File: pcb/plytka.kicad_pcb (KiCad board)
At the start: 2 copper layers, 27 x 78 mm, 51 parts, among them J1 Display, J2 Program, Q3 AO3400A, Q4 AO3400A, SW1 RESET, SW2 USER0, SW3 USER2, SW4 USER3, U1 TPS61022, U2 TP4054, U3 USBLC6-2P6, U4 CH340K

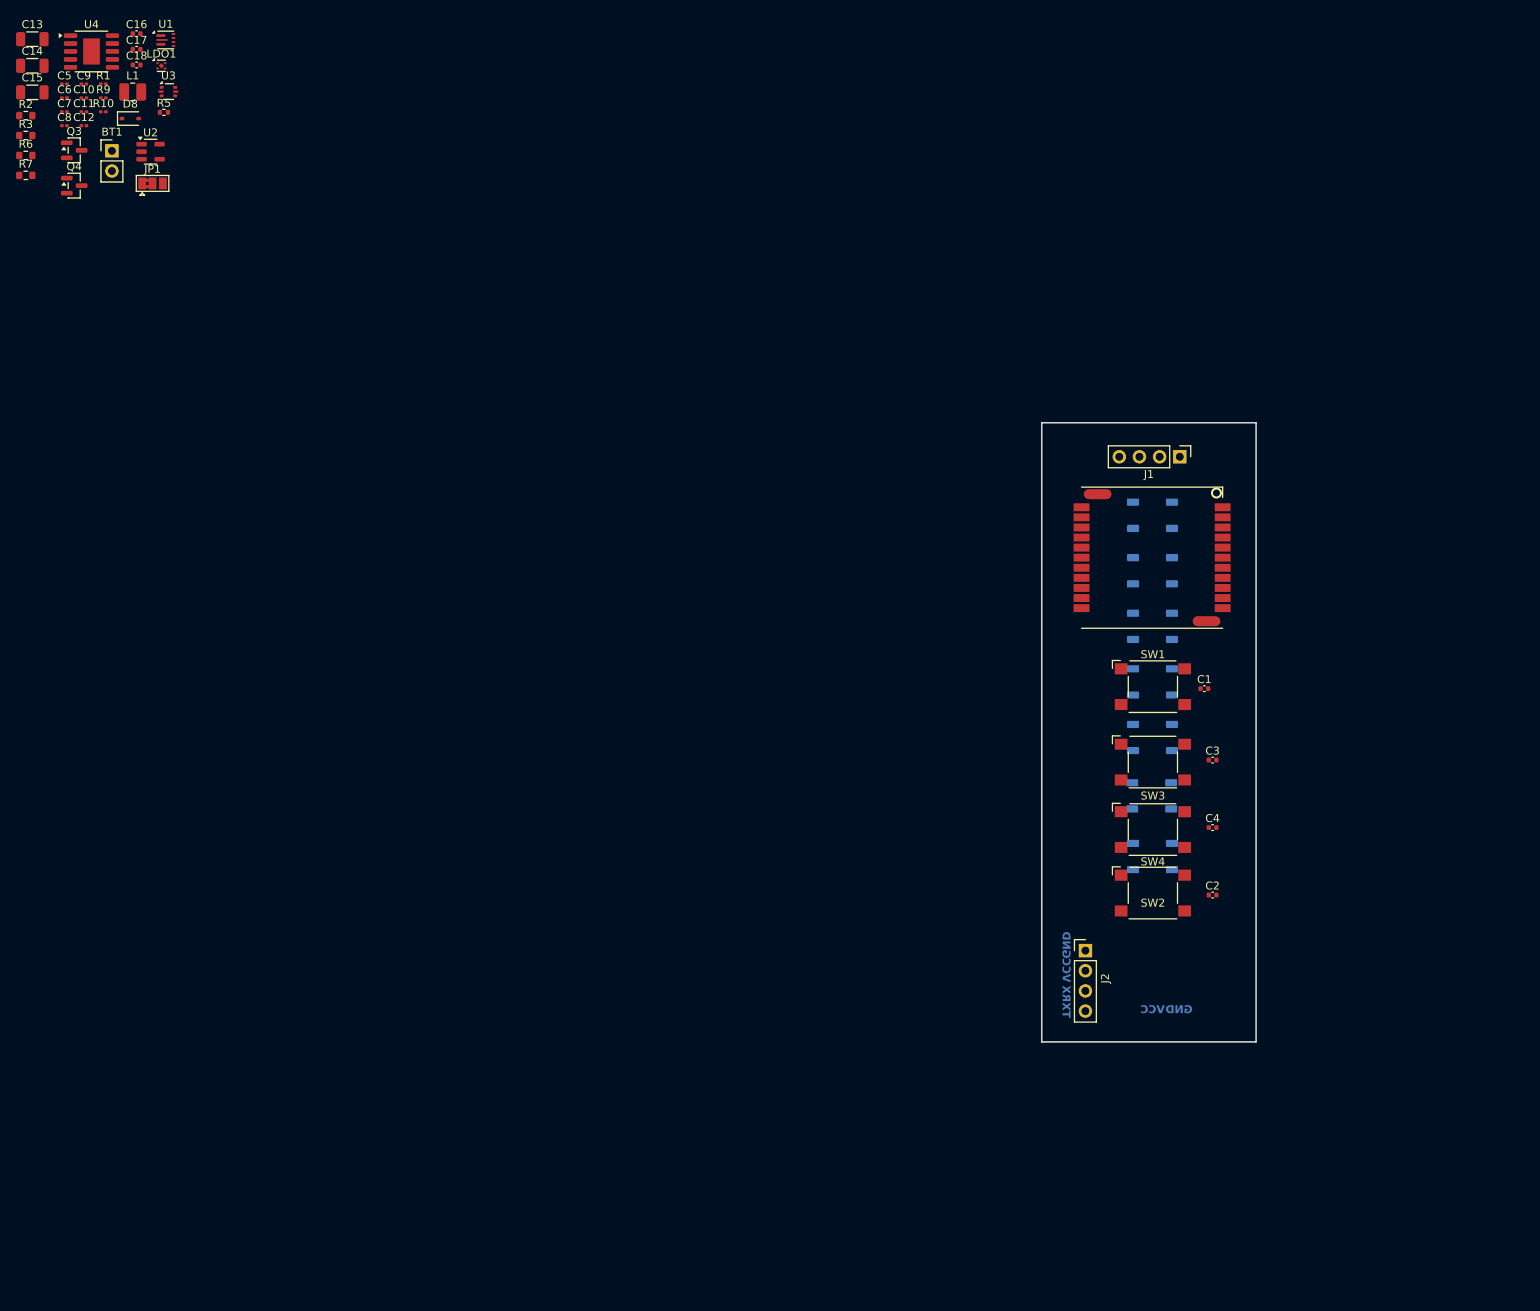
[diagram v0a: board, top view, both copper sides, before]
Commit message: lcsc
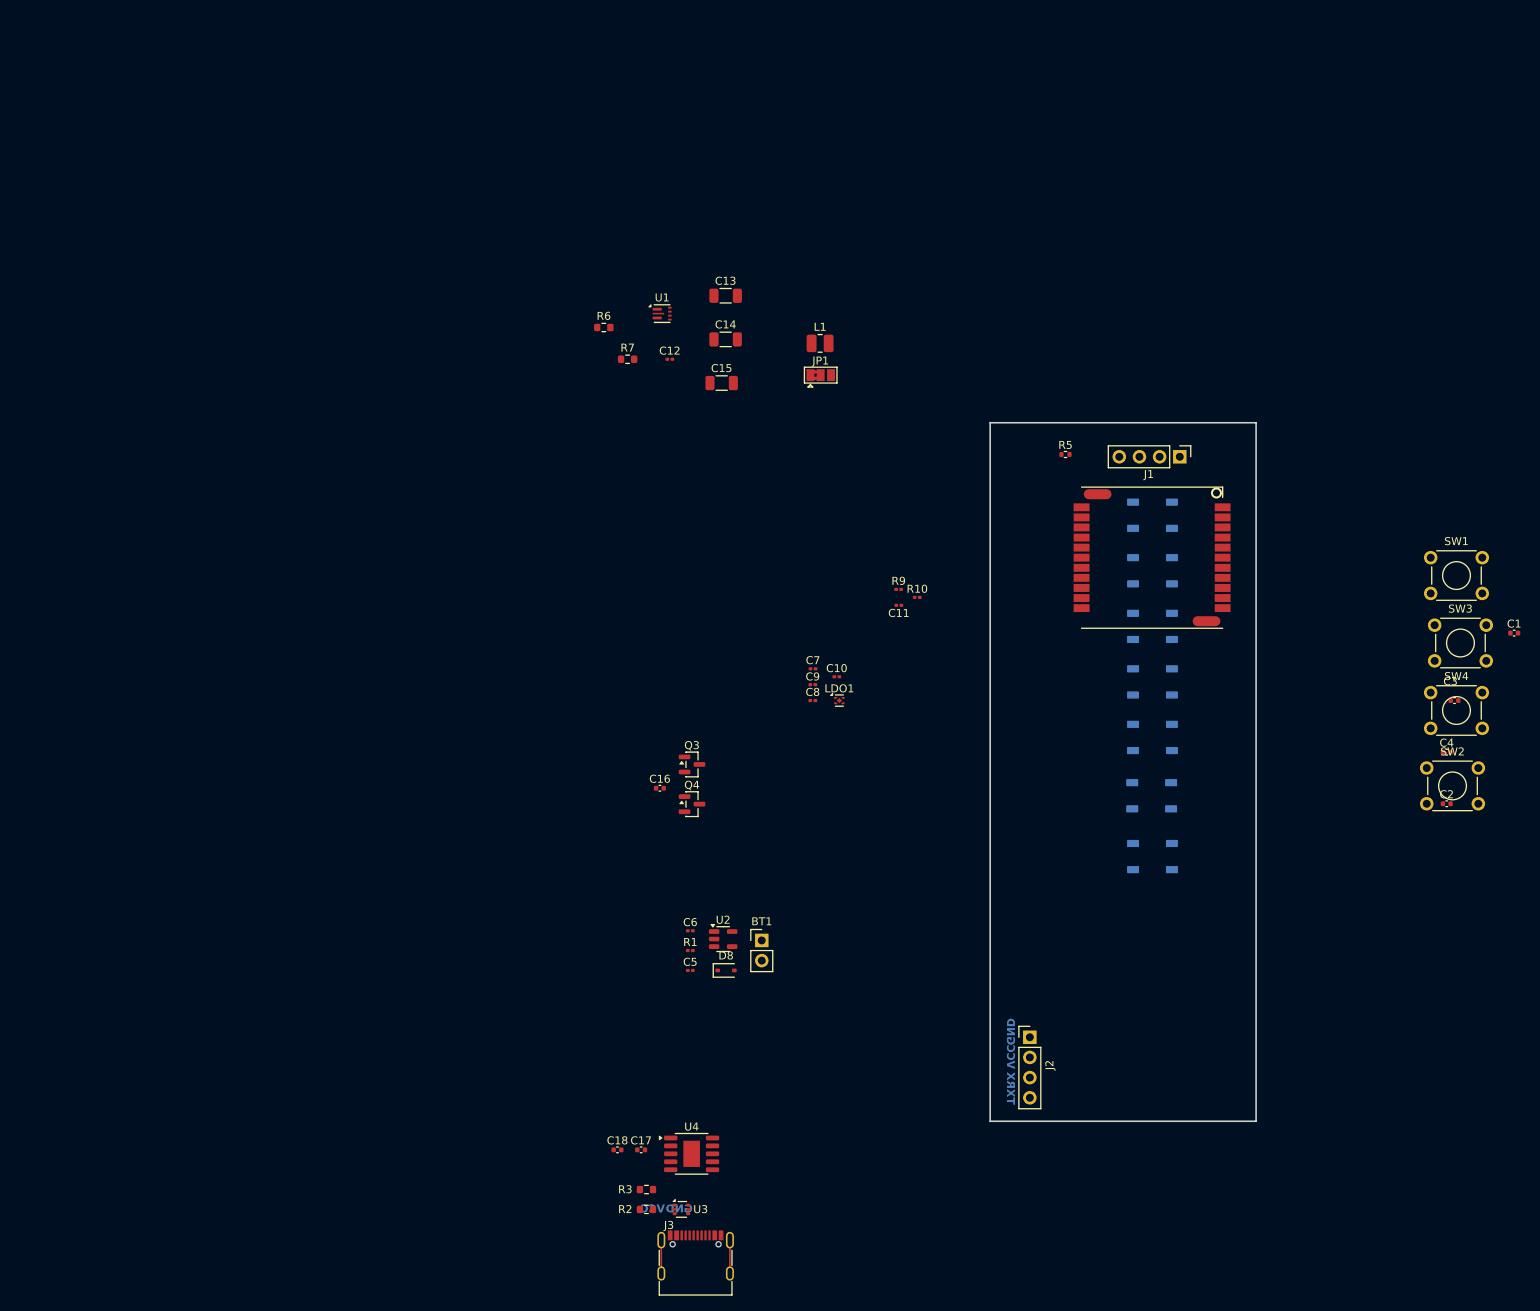
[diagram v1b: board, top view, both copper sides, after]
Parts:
- added J3: USB_C_Receptacle_USB2.0_16P, Connector_USB:USB_C_Receptacle_G-Switch_GT-USB-7010ASV, F.Cu at (85.9, 155.6)
- SW1, SW2, SW3, SW4: footprint Button_Switch_SMD:SW_SPST_Omron_B3FS-100xP -> Button_Switch_THT:SW_TH_Tactile_Omron_B3F-100x
- moved R2 158.4 mm to (79.7, 148.6)
- moved U4 158.1 mm to (85.4, 141.6)
- moved U3 154.9 mm to (84.1, 148.6)
- moved R3 154.1 mm to (79.7, 146.1)
- moved C17 152.5 mm to (79.0, 141.1)
- moved C18 149.5 mm to (76.0, 141.1)
- moved C5 136.7 mm to (85.2, 118.5)
- moved R1 131.9 mm to (85.2, 116.0)
- moved C6 131.3 mm to (85.2, 113.5)
- moved D8 131.0 mm to (89.7, 118.5)
- moved BT1 128.8 mm to (94.2, 114.7)
- moved U2 122.7 mm to (89.4, 114.5)
- moved R5 121.5 mm to (132.5, 53.5)
- moved C11 120.0 mm to (111.5, 72.5)
- moved C10 119.6 mm to (103.7, 81.5)
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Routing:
- net GND: track 0.00 -> 8.40 mm
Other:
- board size 27 x 78 mm -> 33.5 x 88 mm

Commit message: almost finish pcb
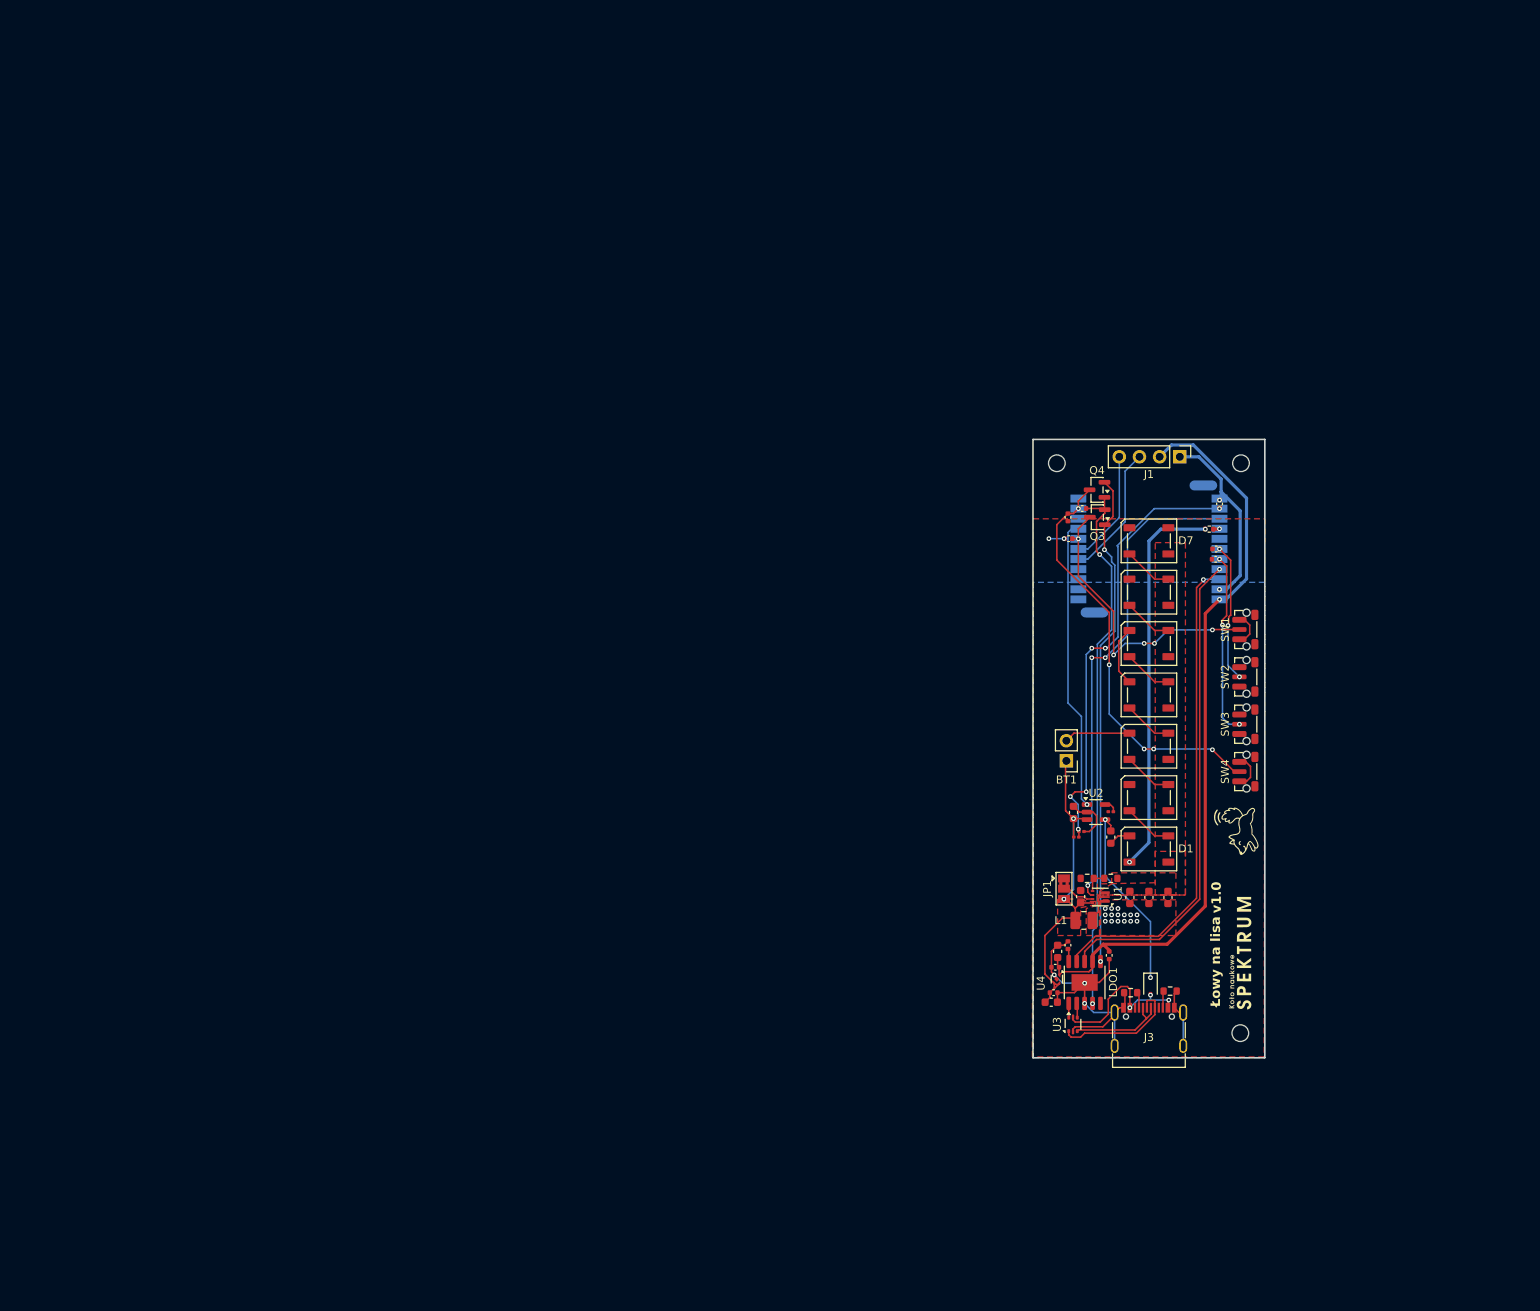
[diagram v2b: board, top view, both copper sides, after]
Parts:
- removed J2: Program, Connector_PinHeader_2.54mm:PinHeader_1x04_P2.54mm_Vertical
- added G*** (x2): LOGO, LOGO, F.Cu at (154.8, 114.5)
- added G***: LOGO, LOGO, F.Cu at (154.1, 100.9)
- added REF**: MountingHole_2.1mm, MountingHole:MountingHole_2.1mm, F.Cu at (154.6, 54.6)
- added REF**: MountingHole_2.1mm, MountingHole:MountingHole_2.1mm, F.Cu at (154.5, 126.4)
- added REF**: MountingHole_2.1mm, MountingHole:MountingHole_2.1mm, F.Cu at (131.4, 54.6)
- C10, C11, C8: footprint Capacitor_SMD:C_0201_0603Metric -> Capacitor_SMD:C_0402_1005Metric
- C12, C5, C6, C7, C9: footprint Capacitor_SMD:C_0201_0603Metric -> Capacitor_SMD:C_0603_1608Metric
- C13, C14, C15: footprint Capacitor_SMD:C_1206_3216Metric -> Capacitor_SMD:C_0603_1608Metric
- D1, D2, D3, D4, D5, D6, D7: moved to F.Cu
- HTCC-AM1: moved to B.Cu
- SW1: renamed from SW2; footprint Button_Switch_THT:SW_TH_Tactile_Omron_B3F-100x -> Button_Switch_SMD:SW_Push_1P1T-MP_NO_Horizontal_Alps_SKRTLAE010
- SW2: renamed from SW3; value USER2 -> USER6; footprint Button_Switch_THT:SW_TH_Tactile_Omron_B3F-100x -> Button_Switch_SMD:SW_Push_1P1T-MP_NO_Horizontal_Alps_SKRTLAE010
- SW3: renamed from SW4; value USER3 -> USER7; footprint Button_Switch_THT:SW_TH_Tactile_Omron_B3F-100x -> Button_Switch_SMD:SW_Push_1P1T-MP_NO_Horizontal_Alps_SKRTLAE010
- SW4: renamed from SW1; footprint Button_Switch_THT:SW_TH_Tactile_Omron_B3F-100x -> Button_Switch_SMD:SW_Push_1P1T-MP_NO_Horizontal_Alps_SKRTLAE010
- moved R6 94.3 mm to (138.2, 106.9), turned to 180 degrees
- moved U1 91.9 mm to (136.9, 109.2), turned to 180 degrees
- moved C13 91.3 mm to (140.6, 109.3), turned to -90 degrees
- moved C14 88.2 mm to (143.0, 109.3), turned to -90 degrees
- moved R7 87.3 mm to (135.2, 106.9), turned to 180 degrees
- moved C15 85.8 mm to (145.4, 109.3), turned to -90 degrees
- moved C12 85.2 mm to (134.4, 109.2), turned to 90 degrees
- moved L1 79.9 mm to (134.8, 112.2)
- moved JP1 71.6 mm to (132.3, 108.2), turned to -90 degrees
- moved R3 70.6 mm to (145.7, 121.1), turned to 180 degrees
- moved R2 66.8 mm to (140.7, 121.3)
- moved C18 66.6 mm to (138.0, 116.6), turned to -90 degrees
- moved Q4 64.6 mm to (136.5, 58.0), turned to 180 degrees
- moved J3 63.9 mm to (143.0, 126.9)
- moved C16 63.8 mm to (134.6, 60.3), turned to 180 degrees
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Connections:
- HTCC-AM1 pad 10: unconnected-(HTCC-AM1-ADC-Pad10) -> BAT_LVL
- U3 pad 1: Net-(J3-D--PadA7) -> Net-(J3-D+-PadA6)
- U3 pad 3: Net-(J3-D+-PadA6) -> Net-(J3-D--PadA7)
- U3 pad 4: D+ -> D-
- U3 pad 6: D- -> D+
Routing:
- net GND: track 8.40 -> 110.2 mm, vias 0 -> 22
- net 3V3: track 0.00 -> 95.0 mm, vias 0 -> 1
- net DTR: track 0.00 -> 68.5 mm, vias 0 -> 2
- net RTS: track 0.00 -> 62.5 mm, vias 0 -> 2
- net UART_TX: track 0.00 -> 61.4 mm, vias 0 -> 1
- net UART_RX: track 0.00 -> 61.1 mm, vias 0 -> 1
- net BOOST_EN: track 0.00 -> 60.9 mm, vias 0 -> 3
- net BAT_LVL: track 0.00 -> 56.2 mm, vias 0 -> 6
- net RESET: track 0.00 -> 52.5 mm, vias 0 -> 5
- net Net-(D1-DIN): track 0.00 -> 49.2 mm, vias 0 -> 2
- net VBAT: track 0.00 -> 43.8 mm, vias 0 -> 2
- net GPIO0: track 0.00 -> 37.5 mm, vias 0 -> 5
- net CHGSTAT: track 0.00 -> 36.8 mm, vias 0 -> 1
- net Net-(D8-K): track 0.00 -> 24.1 mm, vias 0 -> 2
- net GPIO7: track 0.00 -> 23.1 mm, vias 0 -> 3
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- added copper zone on B.Cu, net GND
- added copper zone on F.Cu, net GND
- added copper zone on F.Cu, net LED5V
- added copper zone on F.Cu, net Net-(U1-SW)
- added copper zone on F.Cu, net VBAT
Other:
- board size 33.5 x 88 mm -> 29.2 x 77.9 mm
- board text added: "v1.0"
- board text added: "Łowy na lisa"
- board text removed: "GND"
- board text removed: "RX"
- board text removed: "TX"
- board text removed: "VCC"
